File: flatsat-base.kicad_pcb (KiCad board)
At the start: 2 copper layers, 228.6 x 134.6 mm, 30 parts, among them J1 FFC2B28-24-G, J10 Conn_01x24_Male, J11 Conn_01x10_Male, J12 FFC2B28-10-G, J13 FFC2B28-10-G, J14 Screw_Terminal_01x02, J15 Screw_Terminal_01x02, J2 FFC2B28-10-G, J3 FFC2B28-10-G, J4 FFC2B28-10-G, J5 FFC2B28-10-G, J6 FFC2B28-10-G, J7 FFC2B28-10-G, J8 Conn_02x05_Odd_Even, J9 Conn_02x05_Odd_Even

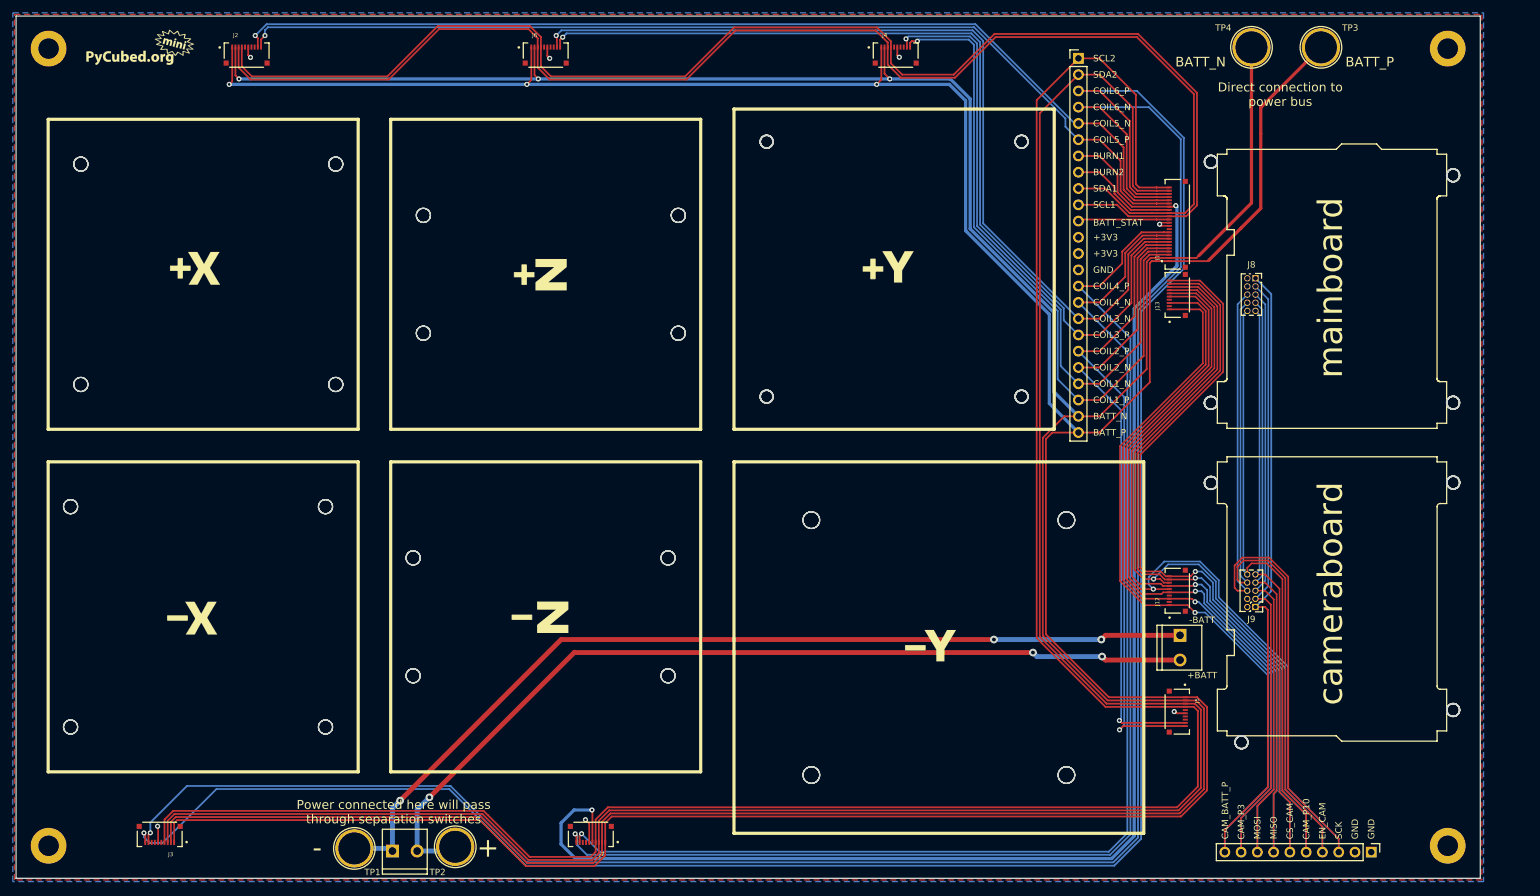
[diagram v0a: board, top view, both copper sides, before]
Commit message: misc changes
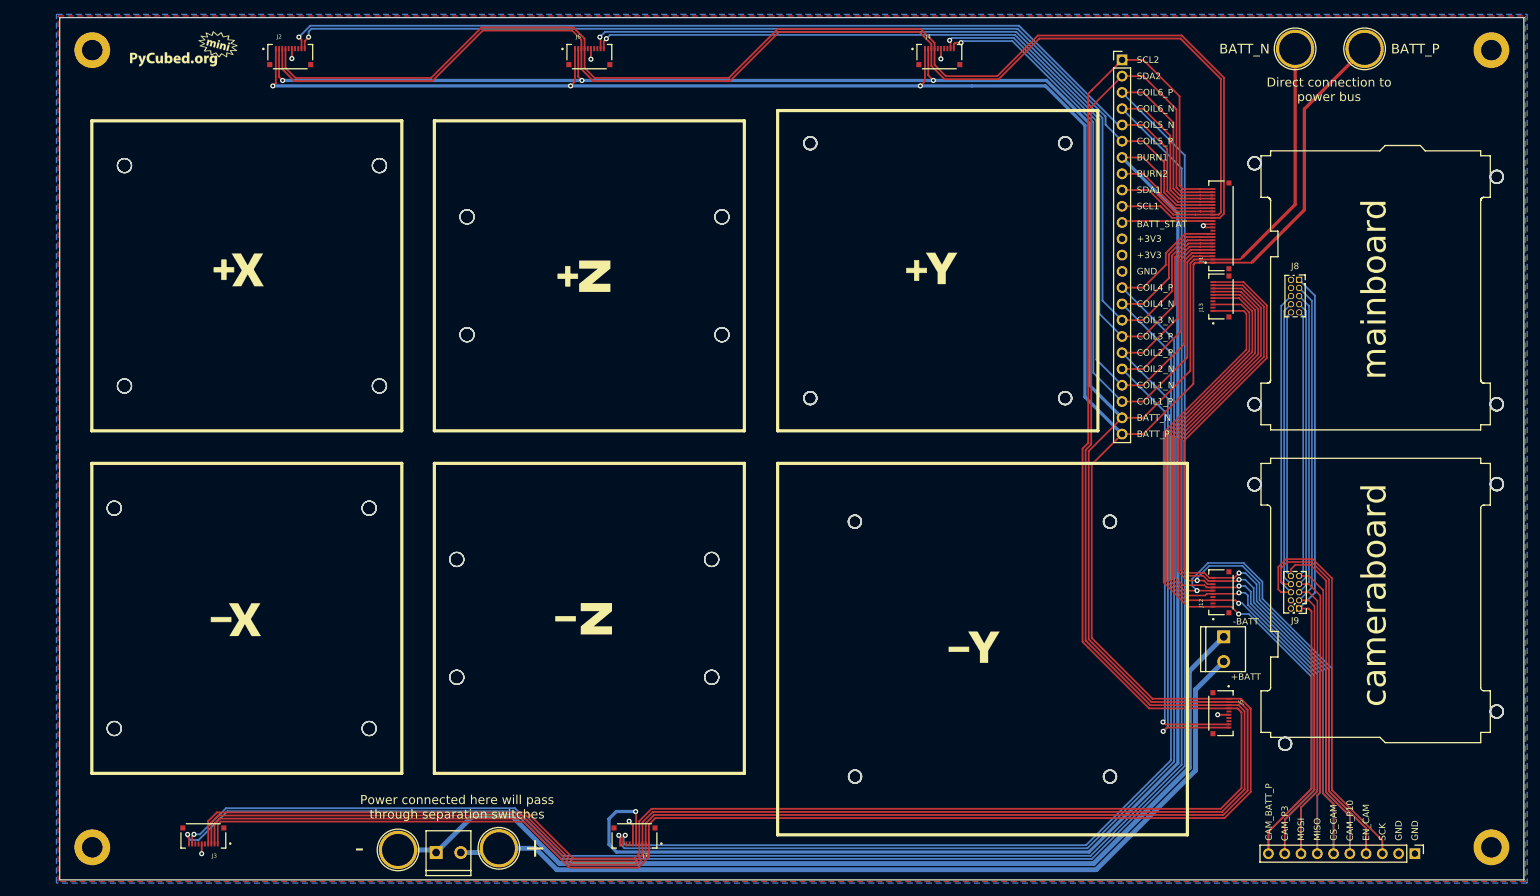
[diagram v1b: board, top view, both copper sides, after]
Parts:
- moved H3 6.82 mm to (259.0, 153.3)
- moved H4 6.82 mm to (259.0, 28.9)
- moved J1 6.82 mm to (216.8, 56.3)
- moved J12 6.82 mm to (216.8, 113.5)
- moved J13 6.82 mm to (216.8, 67.3)
- moved J4 6.82 mm to (172.8, 29.9)
- moved J5 6.82 mm to (216.8, 132.4)
- moved J9 6.82 mm to (229.0, 116.1)
- moved Ref** 6.82 mm to (190.2, 63.9)
- moved TP3 6.82 mm to (239.2, 28.7)
- moved Ref** 6.82 mm to (61.7, 28.2)
- moved H1 6.82 mm to (40.6, 28.9)
- moved H2 6.82 mm to (40.6, 153.3)
- moved J15 6.82 mm to (94.4, 154.2)
- moved J2 6.82 mm to (71.5, 29.9)
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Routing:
- net COIL6_N: track 321.1 -> 297.7 mm
- net COIL6_P: track 327.1 -> 304.9 mm
- net BATT_NOSWITCH_N: track 146.9 -> 158.0 mm, vias 3 -> 0
- net COIL4_P: track 199.3 -> 191.3 mm
- net COIL4_N: track 195.8 -> 189.0 mm
- net BATT_N: track 518.5 -> 521.7 mm
- net SCL1: track 214.2 -> 211.1 mm
- net SDA1: track 214.2 -> 211.2 mm
- net BATT_P: track 530.4 -> 532.6 mm
- net +3V3: track 16.8 -> 15.1 mm
- net BURN1: track 227.4 -> 226.1 mm, vias 2 -> 1
- net BATT_NOSWITCH_P: track 142.4 -> 141.6 mm, vias 3 -> 0
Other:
- outline, holes or cut-outs redrawn
